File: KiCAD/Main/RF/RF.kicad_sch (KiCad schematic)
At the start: 2 parts, among them J9 Conn_Coaxial

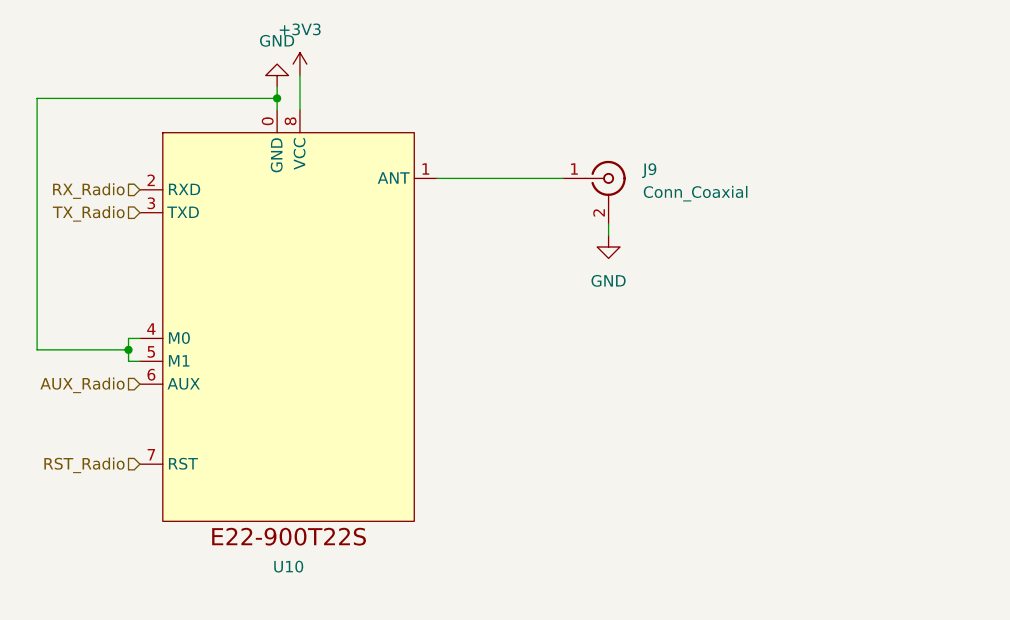
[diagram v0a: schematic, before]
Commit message: Complete layout first draft
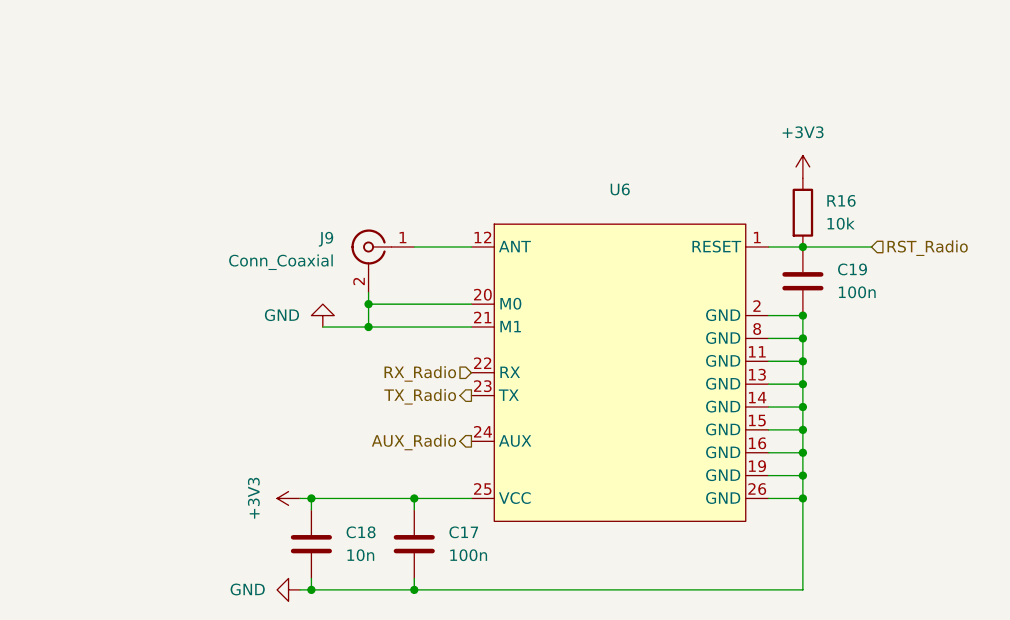
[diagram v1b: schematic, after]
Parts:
- removed U10: ~, E22-900T22S:E22-900T22S, symbol E22-900T22S:E22-900T22S
- added C17, C19: 100n, Capacitor_SMD:C_0603_1608Metric, symbol Device:C
- added C18: 10n, Capacitor_SMD:C_0603_1608Metric, symbol Device:C
- added R16: 10k, Resistor_SMD:R_0603_1608Metric, symbol Device:R
- added U6: ~, E22-900T22S:E22-900T22S, symbol E22-900T22S:E22-900T22S
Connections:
- net +3V3: now also C17.1, C18.1, R16.1, U6.25 (VCC)
- net AUX_Radio: now also U6.24 (AUX)
- net GND: now also C17.2, C18.2, C19.2, U6.11 (GND), U6.13 (GND), U6.14 (GND), U6.15 (GND), U6.16 (GND), U6.19 (GND), U6.2 (GND), U6.20 (M0), U6.21 (M1), U6.26 (GND), U6.8 (GND)
- net RST_Radio: now also C19.1, R16.2, U6.1 (RESET)
- net RX_Radio: now also U6.22 (RX)
- net TX_Radio: now also U6.23 (TX)
- net at J9.1 (In): now also U6.12 (ANT)
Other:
- moved on the sheet: J9
